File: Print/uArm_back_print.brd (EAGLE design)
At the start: 84 x 45 mm, 63 parts, among them IC1 ATmega644PA, IC4 ATTINY24/44/84-SSU, Q1 16MHz

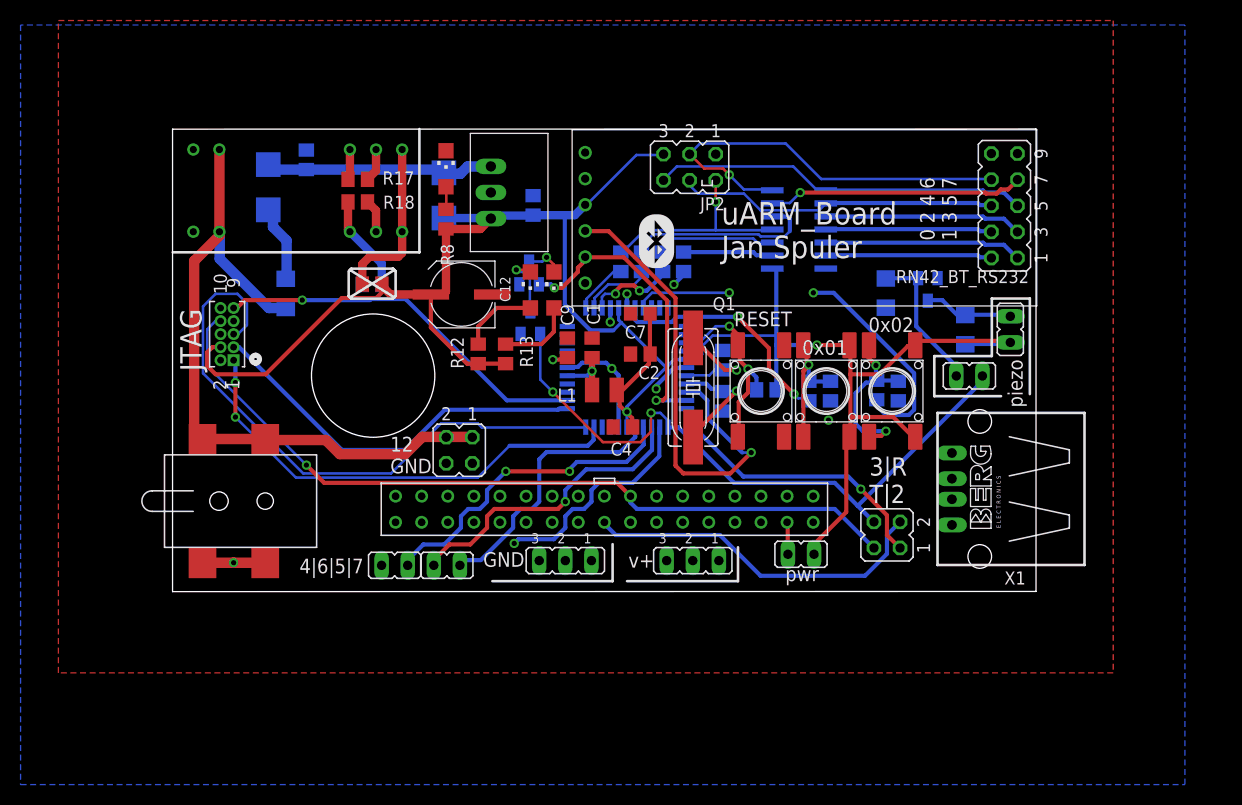
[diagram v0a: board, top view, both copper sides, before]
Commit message: asd
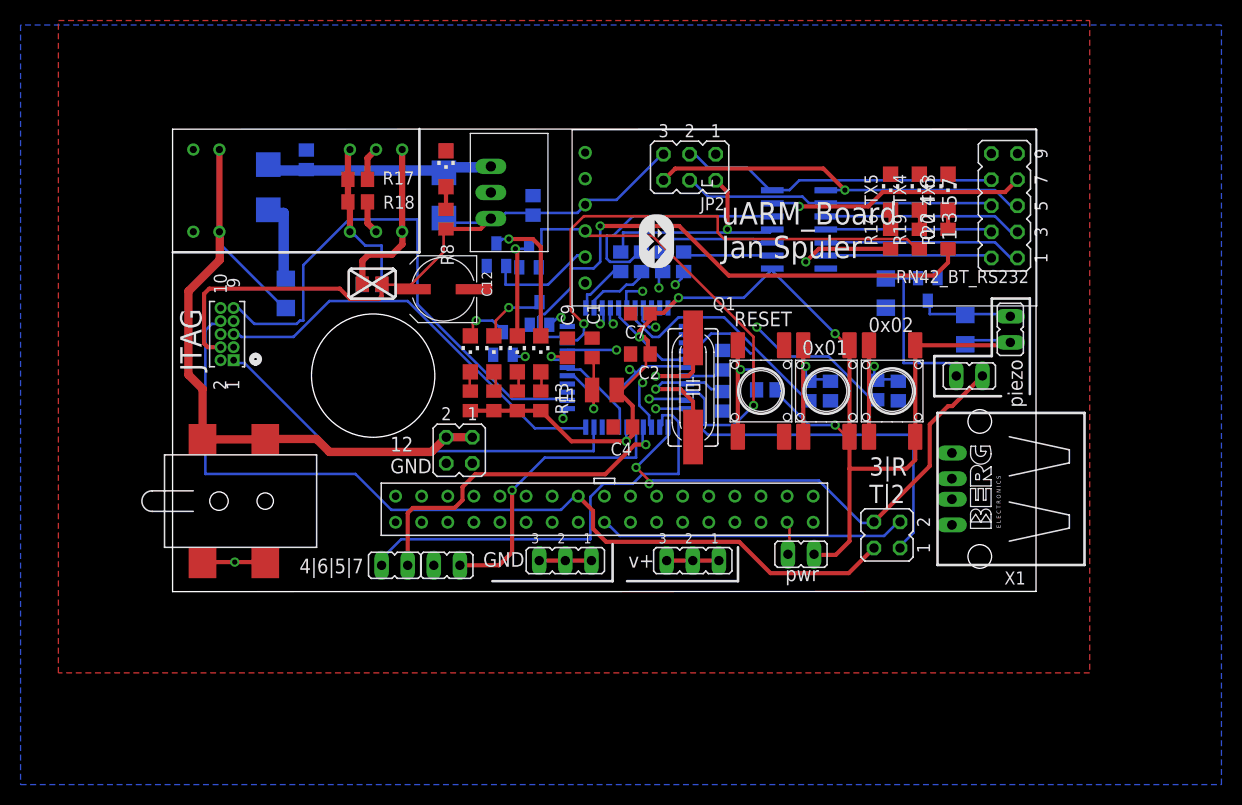
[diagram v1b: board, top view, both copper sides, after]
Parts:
- removed RX, TX: Gruen, led:CHIPLED_1206
- added R14, R15, R16, R19, R20: 1k, rcl:R0805
- added RX1, RX2, TX1, TX2, TX3, TX4, TX5: Gruen, led:CHIPLED_1206
- added V3, V4: PMV20EN, transistor-fet-mit-BSS138:SOT23
- moved V1 6.48 mm to (34.7, 32.6)
- moved R12 5.95 mm to (33.5, 18.5)
- moved R13 5.72 mm to (35.8, 18.5)
- moved V2 3.64 mm to (31.5, 32.8)
- moved C12 1.85 mm to (26.3, 29.4)
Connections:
- new net N$10: R15.1, RX2.A
- new net N$11: R14.1, TX2.A
- new net N$12: TX2.C, V3.3
- new net N$13: R20.2, TX3.A
- new net N$6: R16.2, TX5.A
- new net N$7: R19.2, TX4.A
- new net N$8: RX2.C, V4.3
- net GND: now also TX3.C, TX4.C, TX5.C, V3.2, V4.2
- net N$2: now also TX1.C; no longer TX.C
- net N$3: now also RX1.C; no longer RX.C
- net N$4: now also TX1.A; no longer TX.A
- net N$5: now also RX1.A; no longer RX.A
- net PA5: now also R20.1
- net PA6: now also R19.1
- net PA7: now also R16.1
- net PD0: now also V1.1
- net PD2: now also V3.1
- net PD3: now also V4.1; no longer V1.1
- net TX: now also U$4.15; no longer U$4.19
- net VCC: now also R14.2, R15.2
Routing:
- net PA5: track 0.00 -> 55.2 mm, vias 0 -> 1
- net PA6: track 0.00 -> 49.4 mm, vias 0 -> 1
- net PA7: track 0.00 -> 35.6 mm, vias 0 -> 2
- net PD2: track 28.2 -> 53.3 mm, vias 1 -> 2
- net PC3: track 58.9 -> 41.0 mm
- net PC5: track 36.9 -> 52.6 mm, vias 1 -> 0
- net PB1: track 38.9 -> 27.2 mm
- net DGND: track 38.0 -> 49.2 mm, vias 4 -> 3
- net TX: track 77.8 -> 88.0 mm, vias 1 -> 0
- net N$2: track 3.59 -> 13.5 mm
- net PA6_: track 40.9 -> 31.2 mm, vias 1 -> 0
- net PD4: track 36.2 -> 43.6 mm, vias 1 -> 0
- net N$12: track 0.00 -> 6.59 mm, vias 0 -> 1
- net PD5: track 29.7 -> 35.6 mm
- net N$4: track 7.51 -> 1.90 mm
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
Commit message: geschmeus
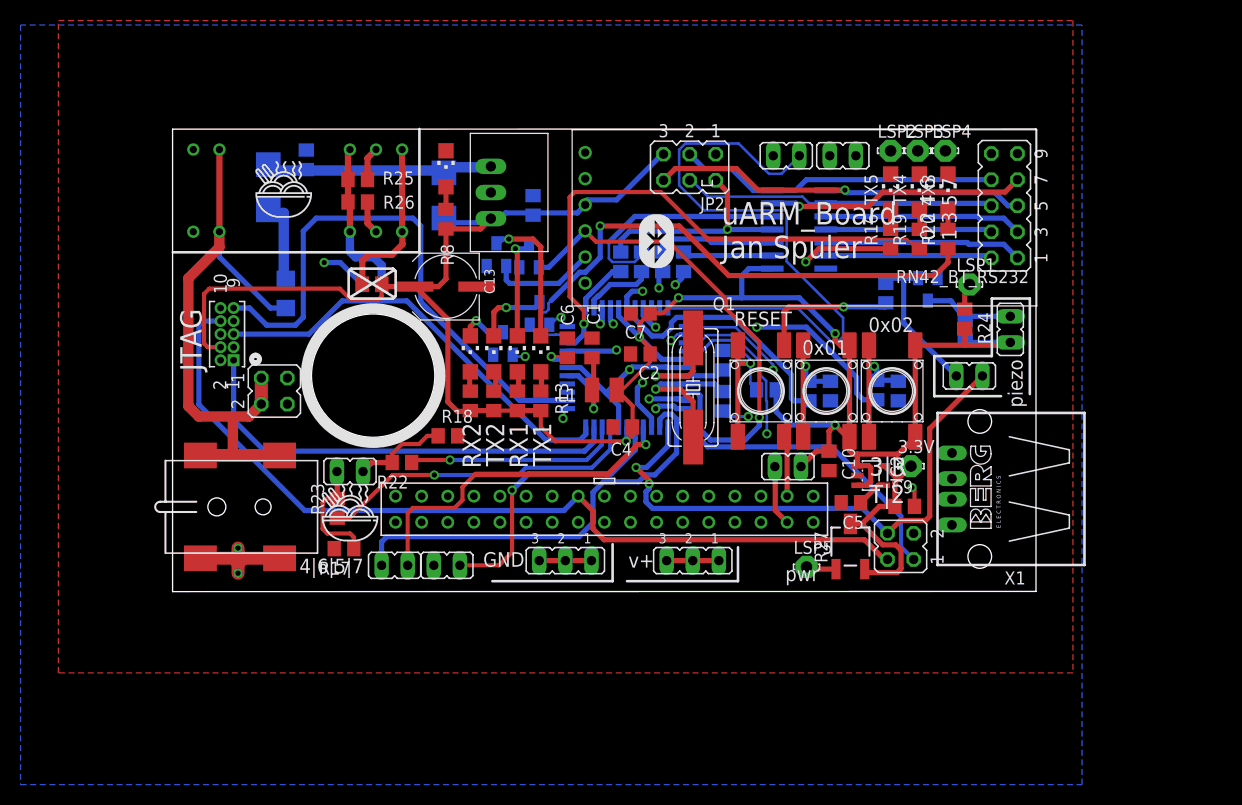
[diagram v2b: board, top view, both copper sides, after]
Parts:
- added 3.3V: 3.3V, solpad:LSP11
- added C10: 1uF, rcl:C0805
- added C13: 100uF, rcl2:UD-6,3X5,8_NICHICON
- added C6: 100nF, rcl:C0805
- added IC2: LP2985-XXDBVR, SmartPrj:SOT23-DBV
- added LSP1, LSP2, LSP3, LSP4, LSP5: LSP11, solpad:LSP11
- added PIEZO-POWER10, PIEZO-POWER8, PIEZO-POWER9: (no value), jumper:JP1
- added R22, R23, R24: 1k, rcl:R0805
- added R25, R26: 1k472, rcl:R0805
- added R27: (no value), pot:3223G
- C11: value 100nF -> 18pF
- C12: value 100uF -> 18pF; device rcl2:UD-6,3X5,8_NICHICON -> rcl:C0805
- C3, C5: value 18pF -> 100nF
- C9: value 100nF -> 1uF
- R1, R2: value 1k -> 100k
- R11, R21: device rcl:R1206 -> rcl:R0805
- R17, R18: value 1k472 -> 1k
- R3, R4: value 100k -> 1k
- R5: value 10k -> 1k
- moved C9 36.3 mm to (71.2, 8.28), turned to 0 degrees
- moved R17 36.0 mm to (16.7, 4.17), turned to 180 degrees
- moved C12 29.3 mm to (53.5, 18.5), flipped to the bottom, turned to 270 degrees
- moved R18 24.4 mm to (26.8, 15.1)
- moved C11 23.8 mm to (53.5, 22.5), turned to 270 degrees
- moved C3 23.8 mm to (35.1, 37.6), turned to 90 degrees
- moved JP3 18.9 mm to (9.89, 19.5), turned to 270 degrees
- moved C5 15.9 mm to (66.0, 8.64), flipped to the top, turned to 180 degrees
- moved U$1 9.72 mm to (4.29, 8.23), turned to 0 degrees
- moved PIEZO-POWER4 8.63 mm to (59.9, 12.1)
- moved R2 2.10 mm to (70.6, 19.5)
- moved R4 2.10 mm to (68.5, 19.6)
- moved R1 2.10 mm to (64.0, 19.5)
- moved R3 2.10 mm to (61.9, 19.5)
- moved JP1 1.73 mm to (70.8, 4.38)
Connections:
- new net 3.3V: 3.3V.MP, C9.1, IC2.5, R27.2, R27.3
- new net N$14: PIEZO-POWER10.2, R18.1, R22.2
- new net N$15: PIEZO-POWER10.1, R17.1, R23.2
- new net N$17: LSP5.MP, R27.1
- new net N$18: LSP1.MP, R24.1
- new net N$70: C5.1, IC2.4
- net DGND: now also R25.1, R26.1; no longer R17.1, R18.1
- net GND: now also C10.2, C11.1, C12.2, C13.-, C3.2, C6.1, C9.2, IC2.2, LSP2.MP, LSP3.MP, LSP4.MP, R1.1, R17.2, R18.2, R2.1; no longer C11.2, C12.-, C3.1, C9.1, R3.1, R4.1
- net N$16: now also R26.2; no longer R18.2
- net N$36: now also C12.1; no longer C5.1
- net N$37: now also C11.2; no longer C3.2
- net N$38: now also C6.2; no longer C9.2
- net N$85: now also R25.2; no longer R17.2
- net PB0: now also R3.1; no longer R1.1
- net PB1: now also R4.1; no longer R2.1
- net PB4: now also PIEZO-POWER9.1
- net PB5: now also PIEZO-POWER9.2
- net PB6: now also PIEZO-POWER8.1
- net PB7: now also PIEZO-POWER8.2
- net PC0: now also R23.1
- net PC1: now also R22.1
- net VCC: now also C10.1, C13.+, C3.1, IC2.1, IC2.3, R24.2; no longer C11.1, C12.+
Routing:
- net PB4: track 0.00 -> 62.0 mm
- net PB7: track 0.00 -> 51.8 mm, vias 0 -> 1
- net PB6: track 0.00 -> 38.8 mm, vias 0 -> 1
- net PC0: track 0.00 -> 31.5 mm, vias 0 -> 1
- net PB5: track 0.00 -> 31.4 mm, vias 0 -> 1
- net GND: track 0.00 -> 28.8 mm, vias 0 -> 4
- net 3.3V: track 0.00 -> 22.0 mm
- net PC1: track 0.00 -> 20.9 mm, vias 0 -> 1
- net VCC: track 204.6 -> 217.3 mm
- net RX: track 80.7 -> 93.2 mm
- net N$15: track 0.00 -> 11.3 mm
- net N$14: track 0.00 -> 9.23 mm
- net +12V: track 66.9 -> 59.2 mm
- net PD3: track 66.4 -> 71.7 mm
- net PA6: track 49.4 -> 52.4 mm
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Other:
- board text added: "RX1"
- board text added: "RX2"
- board text added: "TX1"
- board text added: "TX2"
- board text removed: "12 GND"
- board text removed: "C:/Users/Jan Spuler/OneDrive - MSW-Winterthur/Desktop/bt.bmp"

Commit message: lol
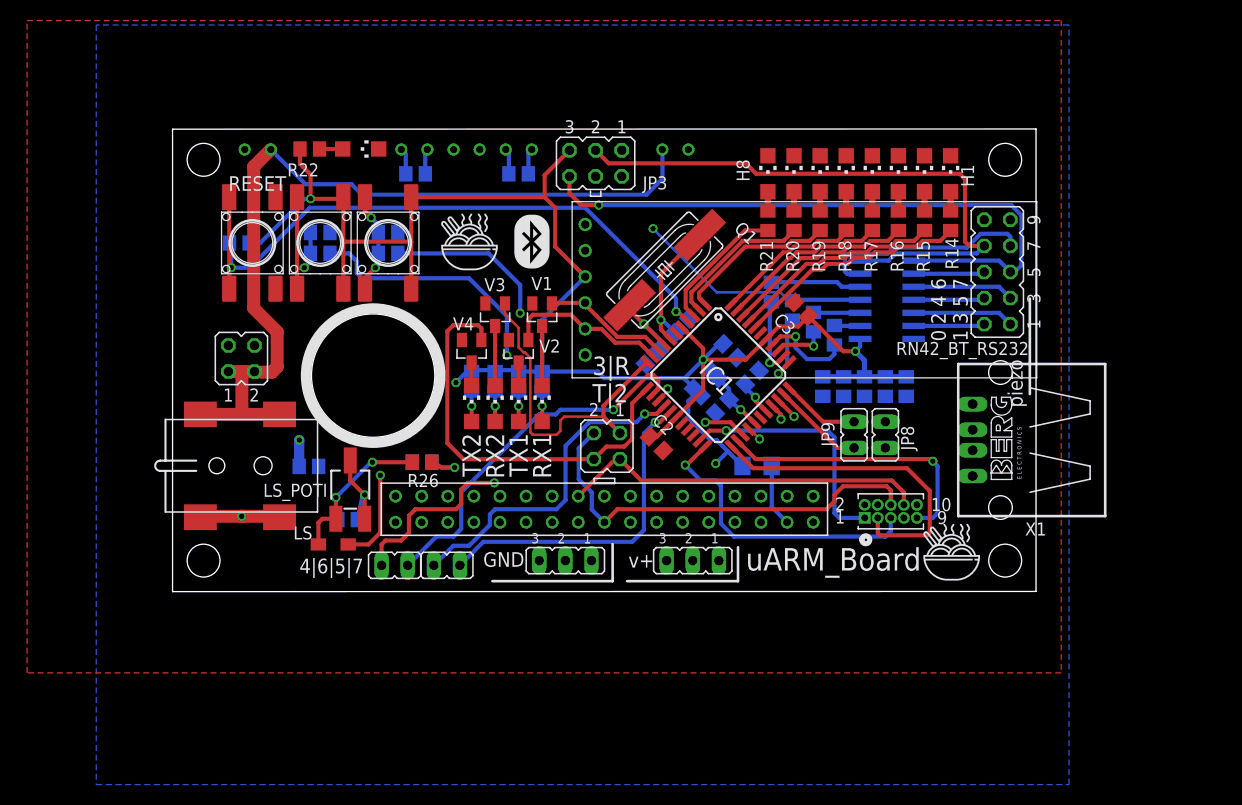
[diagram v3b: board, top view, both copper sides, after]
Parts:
- removed +5V-POWER, RX1, RX2, TX1, TX2, TX3, TX4, TX5: Gruen, led:CHIPLED_1206
- removed 0_OHM_A: 0 Ohm, rcl:R0805
- removed 3.3V: 3.3V, solpad:LSP11
- removed 5V_DC: RECOM_DCDC, DCDC:RECOM_DCDC
- removed D1, D2: MBRS130LT3, diode:SMB
- removed LSP1, LSP2, LSP3, LSP4, LSP5: LSP11, solpad:LSP11
- removed PIEZO-POWER1, PIEZO-POWER10, PIEZO-POWER2, PIEZO-POWER4, PIEZO-POWER8, PIEZO-POWER9: (no value), jumper:JP1
- removed R27: (no value), pot:3223G
- removed U$2, U$3: DCDC, untitled:1X2,3_2.54MM
- removed V12: PMV20EN, transistor-fet-mit-BSS138:SOT23
- added H1, H10, H11, H12, H13, H2, H3, H4, H5, H6, H7, H8, H9: Gruen, led:CHIPLED_1206
- added IC3: DCDC, untitled:1X2,3_2.54MM
- added JP8, JP9: (no value), jumper:JP1
- added LS: ALS-PT17, Lichtsensor:SOD232-W
- added LS_POTI: 25k, pot:3223G
- C11: value 18pF -> 1uF
- C13: value 100uF -> 18pF; device rcl2:UD-6,3X5,8_NICHICON -> rcl:C0805
- C6, C7, C8: value 100nF -> 1uF
- IC2: value LP2985-XXDBVR -> ATTINY24/44/84-SSU; device SmartPrj:SOT23-DBV -> attiny24_44_84:SOIC14
- IC4: value ATTINY24/44/84-SSU -> DCDC; device attiny24_44_84:SOIC14 -> untitled:1X2,3_2.54MM
- JP2: device jumper:JP3Q -> jumper:JP2Q
- JP3: device jumper:JP2Q -> jumper:JP3Q
- R1, R2: value 100k -> 1k
- R10, R6, R7, R9: value 150R -> 1k
- R23, R24: value 1k -> 1k472
- R25: value 1k472 -> 10k
- R26: value 1k472 -> 100k
- moved JTAG 70.4 mm to (72.4, 8.43), turned to 0 degrees
- moved R17 60.5 mm to (68.1, 36.1), turned to 270 degrees
- moved C8 58.6 mm to (67.3, 19.9)
- moved R24 55.3 mm to (23.6, 40.6), flipped to the bottom, turned to 180 degrees
- moved IC4 54.5 mm to (7.00, 43.0), flipped to the top, turned to 0 degrees
- moved R5 53.2 mm to (6.48, 33.9)
- moved R1 52.0 mm to (14.4, 34.9), turned to 0 degrees
- moved R2 52.0 mm to (21.0, 34.9), turned to 0 degrees
- moved RESET 51.5 mm to (7.75, 33.9)
- moved S1 51.3 mm to (14.4, 33.9)
- moved S2 51.1 mm to (21.0, 33.9)
- moved R3 49.4 mm to (14.4, 32.9), turned to 0 degrees
- moved R4 49.4 mm to (21.0, 32.9), turned to 0 degrees
- moved F1 48.8 mm to (56.9, 12.2), turned to 0 degrees
- moved R14 47.8 mm to (75.7, 36.1)
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- renumbered PIEZO-POWER3 to JP4, PIEZO-POWER5 to JP5, UART_ROBO1 to JP6, UART_ROBO2 to JP7
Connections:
- removed net 3.3V: 3.3V.MP, C9.1, IC2.5, R27.2, R27.3
- removed net N$13: R20.2, TX3.A
- removed net N$46: PIEZO-POWER2.2, R21.2, V12.3
- removed net N$70: C5.1, IC2.4
- removed net N$75: 5V_DC.IN, C8.1, D1.C, D2.C
- removed net PD8: PIEZO-POWER1.2, R11.1, V12.1
- new net N$19: H6.A, R19.1
- new net N$20: H7.A, R20.1
- new net N$23: H8.A, R21.1
- net +12V: now also IC3.V_IN, IC4.V_IN, JP2.1, JP2.3; no longer F1.1, JP3.1, JP3.3, U$2.V_IN, U$3.V_IN
- net +5V: now also IC3.V_OUT, IC4.V_OUT; no longer 0_OHM_A.2, U$2.V_OUT, U$3.V_OUT
- net DGND: now also IC3.GND, IC4.GND, JP2.2, JP2.4, R23.1, R24.1; no longer IC1.18, IC1.28, IC1.39, IC1.6, JP3.2, JP3.4, R25.1, R26.1, U$2.GND, U$3.GND
- net GND: now also C10.1, C13.1, C5.1, C7.1, C8.1, C9.1, H1.C, H13.C, H2.C, H3.C, H4.C, H5.C, H6.C, H7.C, H8.C, IC1.18, IC1.28, IC1.39, IC1.6, IC2.14, JP3.1, R25.1; no longer +5V-POWER.C, 5V_DC.GND, C10.2, C13.-, C5.2, C7.2, C8.2, C9.2, IC2.2, IC4.14, JP2.1, LSP2.MP, LSP3.MP, LSP4.MP, R11.2, R17.2, R18.2, TX3.C, TX4.C, TX5.C, V12.2
- net N$1: now also F1.1; no longer PIEZO-POWER4.2
- net N$10: now also H12.A, R13.1; no longer R15.1, RX2.A
- net N$11: now also H11.A, R12.1; no longer R14.1, TX2.A
- net N$12: now also H11.C; no longer TX2.C
- net N$14: now also H2.A, R15.1; no longer PIEZO-POWER10.2, R18.1, R22.2
- net N$15: now also H3.A, R16.1; no longer PIEZO-POWER10.1, R17.1, R23.2
- net N$16: now also IC3.TRIM, R23.2; no longer R26.2, U$3.TRIM
- net N$17: now also H4.A, R17.1; no longer LSP5.MP, R27.1
- net N$18: now also H5.A, R18.1; no longer LSP1.MP, R24.1
- net N$2: now also H10.C; no longer TX1.C
- net N$3: now also H9.C; no longer RX1.C
- net N$37: now also C13.2; no longer C11.2
- net N$38: now also C5.2; no longer C6.2
- net N$4: now also H10.A, R11.1; no longer R13.1, TX1.A
- net N$5: now also H9.A, R10.1; no longer R12.1, RX1.A
- net N$6: now also LS.E, LS_POTI.1, R26.2; no longer R16.2, TX5.A
- net N$60: now also H13.A, R22.1; no longer +5V-POWER.A, R8.1
- net N$7: now also LS_POTI.2, LS_POTI.3, R25.2; no longer R19.2, TX4.A
- net N$8: now also H12.C; no longer RX2.C
- net N$85: now also IC4.TRIM, R24.2; no longer R25.2, U$2.TRIM
- net N$9: now also H1.A, R14.1; no longer D1.A, F1.2
- net PA0_: now also IC2.13; no longer IC4.13
- net PA1_: now also IC2.12; no longer IC4.12
- net PA2: now also R8.1; no longer R9.1
- net PA2_: now also IC2.11; no longer IC4.11
- net PA3: now also R9.1; no longer R10.1
- net PA3_: now also IC2.10; no longer IC4.10
- net PA4: now also JP9.2
- net PA4_: now also IC2.9, JP3.4; no longer IC4.9, JP2.4
- net PA5: now also JP9.1; no longer R20.1
- net PA5_: now also IC2.8, JP3.6; no longer IC4.8, JP2.6
- net PA6: now also JP8.2; no longer R19.1
- net PA6_: now also IC2.7, JP3.3; no longer IC4.7, JP2.3
- net PA7: now also C11.2, JP8.1, R26.1; no longer R16.1
- net PA7_: now also IC2.6; no longer IC4.6
- net PB0: now also R14.2; no longer R3.1
- net PB0_: now also IC2.2; no longer IC4.2
- net PB1: now also R15.2; no longer R4.1
- net PB1_: now also IC2.3; no longer IC4.3
- net PB2: now also R16.2
- net PB2_: now also IC2.5, R8.2; no longer IC4.5, R9.2
- net PB3: now also R17.2
- net PB3_: now also IC2.4, JP3.2, R9.2; no longer IC4.4, JP2.2, R10.2
- net PB4: now also R18.2; no longer PIEZO-POWER9.1
- net PB5: now also R19.2; no longer PIEZO-POWER9.2
- net PB6: now also R20.2; no longer PIEZO-POWER8.1
- net PB7: now also R21.2; no longer PIEZO-POWER8.2
- net PC0: no longer R23.1
- net PC1: no longer R22.1
- net PC6: now also R4.1
- net PC7: now also R3.1
- net PD3: no longer PIEZO-POWER1.1
- net PD4: now also JP4.2; no longer JP4.1
- net PD5: now also JP4.1; no longer JP5.2
- net PD6: now also JP5.2; no longer JP4.2
- net VCC: now also C10.2, C6.2, C7.2, C8.2, C9.2, F1.2, JP3.5, LS.C, R10.2, R11.2, R22.2; no longer 0_OHM_A.1, 5V_DC.OUT, C10.1, C13.+, C7.1, D2.A, IC2.3, IC4.1, JP2.5, PIEZO-POWER2.1, PIEZO-POWER4.1, R14.2, R15.2, R21.1, R24.2, R8.2
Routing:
- net PC7: track 0.00 -> 53.8 mm, vias 0 -> 2
- net RX: track 93.2 -> 41.7 mm
- net TX: track 85.4 -> 35.7 mm
- net PB4: track 62.0 -> 14.2 mm
- net PA5: track 53.6 -> 9.01 mm, vias 1 -> 0
- net RESET: track 20.8 -> 64.1 mm, vias 1 -> 2
- net PC6: track 0.00 -> 42.6 mm, vias 0 -> 2
- net PA6: track 52.4 -> 12.3 mm
- net PB7: track 51.8 -> 13.2 mm, vias 1 -> 0
- net DGND: track 51.9 -> 15.6 mm, vias 4 -> 2
- net PD0: track 47.6 -> 12.4 mm, vias 1 -> 0
- net PC0: track 31.5 -> 0.00 mm, vias 1 -> 0
- net PD3: track 71.7 -> 40.7 mm, vias 3 -> 0
- net GND: track 28.8 -> 0.00 mm, vias 4 -> 0
- net PC5: track 54.0 -> 27.3 mm, vias 0 -> 1
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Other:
- board text added: "uARM_Board"
- board text removed: "0x01"
- board text removed: "0x02"
- board text removed: "pwr"
- board text removed: "uARM_Board Jan Spuler"

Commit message: yeees
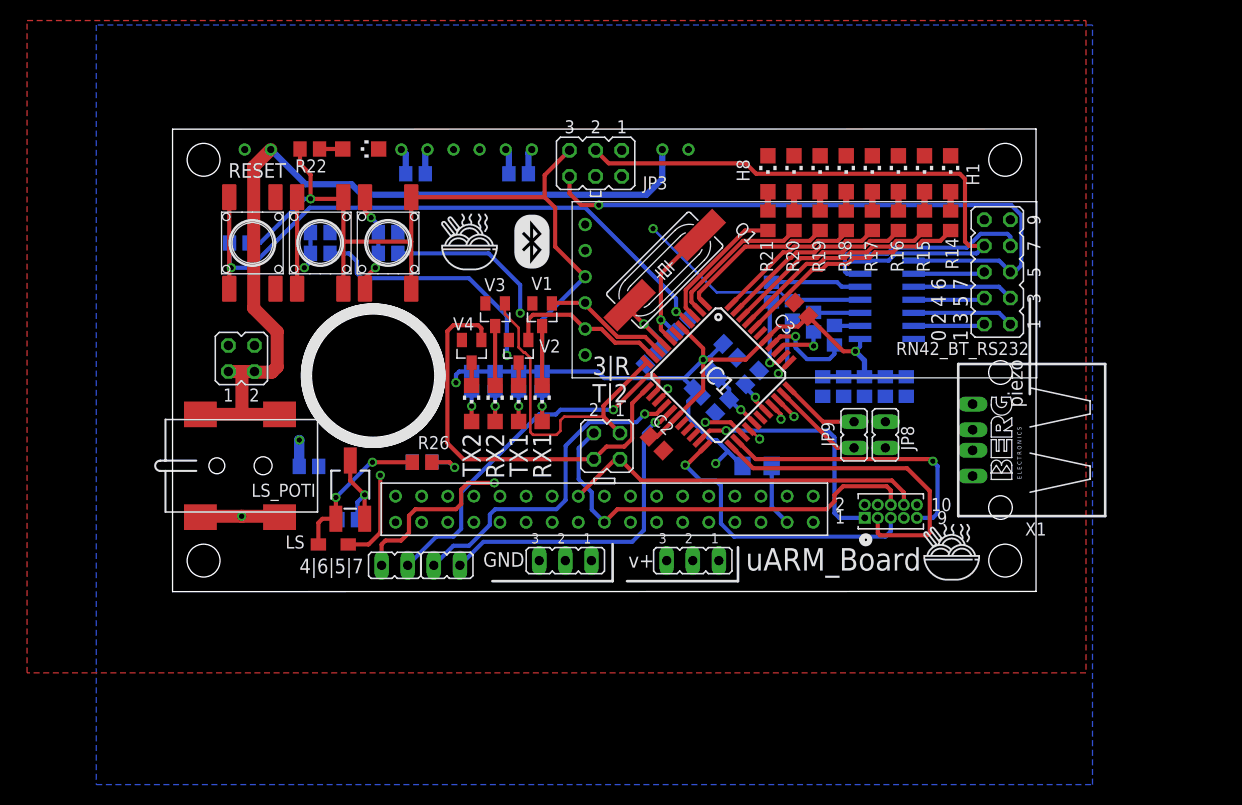
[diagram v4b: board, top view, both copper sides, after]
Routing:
- net VCC: track 208.8 -> 204.9 mm
- net N$22: track 11.0 -> 9.98 mm
- net N$21: track 14.1 -> 13.4 mm
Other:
- board text added: "Jan Spuler 18.02.2020"
- board text added: "R10"
- board text added: "R12"
- board text added: "R13"
